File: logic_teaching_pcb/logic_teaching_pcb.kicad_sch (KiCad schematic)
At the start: 88 parts, among them J1 Conn_01x02, J13 Conn_01x02, J14 Conn_01x01, J15 Conn_01x02, J16 Conn_01x01, J17 Conn_01x01, J18 Conn_01x01, J2 Conn_01x02, J25 Conn_01x02, J26 Conn_01x01, J27 Conn_01x02, J28 Conn_01x01, J29 Conn_01x02, J3 Conn_01x02, J30 Conn_01x02, J31 Conn_01x02, J32 Conn_01x01, J33 Conn_01x02, J34 Conn_01x01, J35 Conn_01x02, J36 Conn_01x01, J37 Conn_01x02, J38 Conn_01x01, J39 Conn_01x02, J4 Conn_01x02, J40 Conn_01x01, J41 Conn_01x02, J42 Conn_01x01, J43 Conn_01x02, J44 Conn_01x01, J45 Conn_01x01, J46 Conn_01x02, J47 Conn_01x01, J48 Conn_01x02, J49 Conn_01x01, J5 Conn_01x01, J50 Conn_01x02, J51 Conn_01x01, J52 Conn_01x02, J53 Conn_01x01, J54 Conn_01x02, J55 Conn_01x01, J56 Conn_01x01, J57 Conn_01x01, J58 Conn_01x01, J59 Conn_01x02, J6 Conn_01x01, J60 Conn_01x02, J61 Conn_01x02, J62 Conn_01x02, J63 Conn_01x01, J64 Conn_01x01, J65 Conn_01x01, J66 Conn_01x01, J7 Conn_01x01, J8 Conn_01x01, J9 Conn_01x01, SW1 SW_SPDT, SW5 SW_Push, SW6 SW_Push, SW7 SW_Push, SW8 SW_Push, U1 74HC00, U2 74HC00

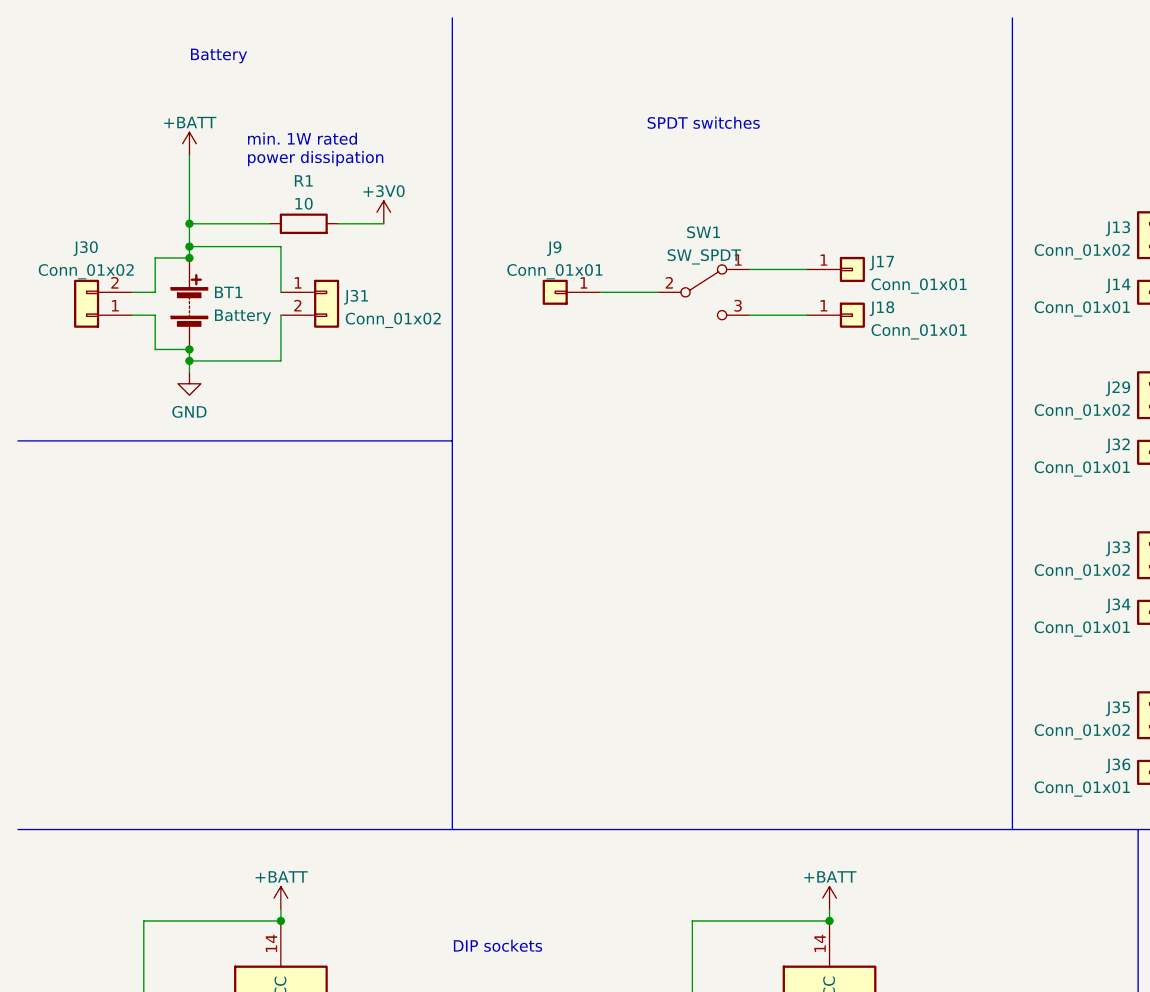
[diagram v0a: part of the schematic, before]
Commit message: finish first PCB draft
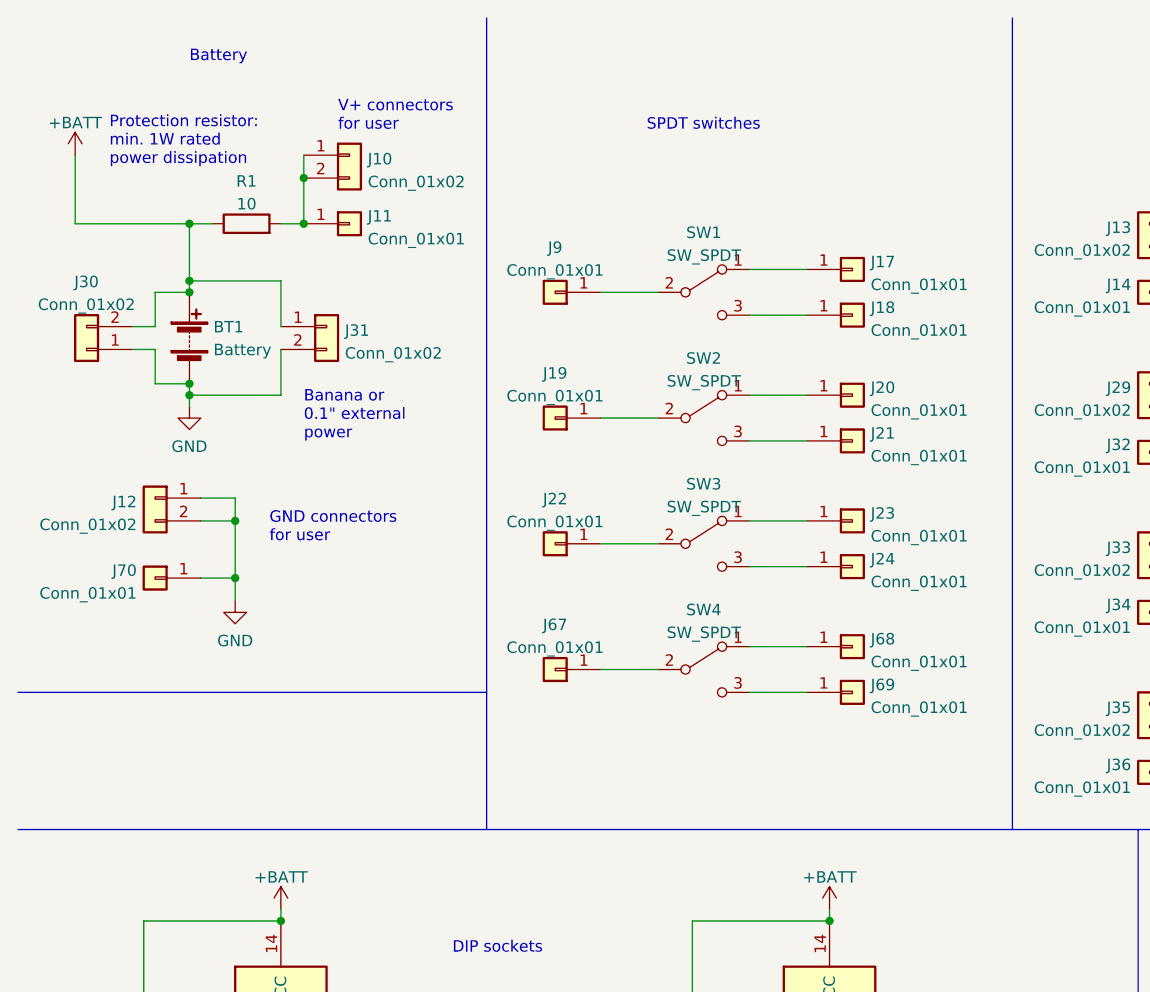
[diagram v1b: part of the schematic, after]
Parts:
- added J10, J12: Conn_01x02, Connector_PinHeader_2.54mm:PinHeader_1x02_P2.54mm_Vertical, symbol Connector_Generic:Conn_01x02
- added J11, J70: Conn_01x01, Connector:Banana_Jack_1Pin, symbol Connector_Generic:Conn_01x01
- added J19, J20, J21, J22, J23, J24, J67, J68, J69: Conn_01x01, Connector_PinHeader_2.54mm:PinHeader_1x01_P2.54mm_Vertical, symbol Connector_Generic:Conn_01x01
- added SW2, SW3, SW4: SW_SPDT, Button_Switch_THT:SW_Slide_1P2T_CK_OS102011MS2Q, symbol Switch:SW_SPDT
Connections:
- net GND: now also J12.1 (Pin_1), J12.2 (Pin_2), J70.1 (Pin_1)
- net +3V0: no longer names the net of R1.2
- net +3V0: now also J10.1 (Pin_1), J10.2 (Pin_2), J11.1 (Pin_1)
- new net: J19.1 (Pin_1), SW2.2 (B)
- new net: J21.1 (Pin_1), SW2.3 (C)
- new net: J22.1 (Pin_1), SW3.2 (B)
- new net: J69.1 (Pin_1), SW4.3 (C)
- new net: J67.1 (Pin_1), SW4.2 (B)
- new net: J20.1 (Pin_1), SW2.1 (A)
- new net: J24.1 (Pin_1), SW3.3 (C)
- new net: J68.1 (Pin_1), SW4.1 (A)
- new net: J23.1 (Pin_1), SW3.1 (A)
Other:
- note added: "Banana or 0.1" external power"
- note added: "GND connectors for user"
- note added: "Protection resistor: min. 1W rated power dissipation"
- note added: "V+ connectors for user"
- note removed: "min. 1W rated power dissipation"
- moved on the sheet: BT1, J30, J31, R1
